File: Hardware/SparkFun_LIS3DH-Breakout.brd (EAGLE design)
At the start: 15.2 x 15.2 mm, 15 parts, among them U2 LIS3DH

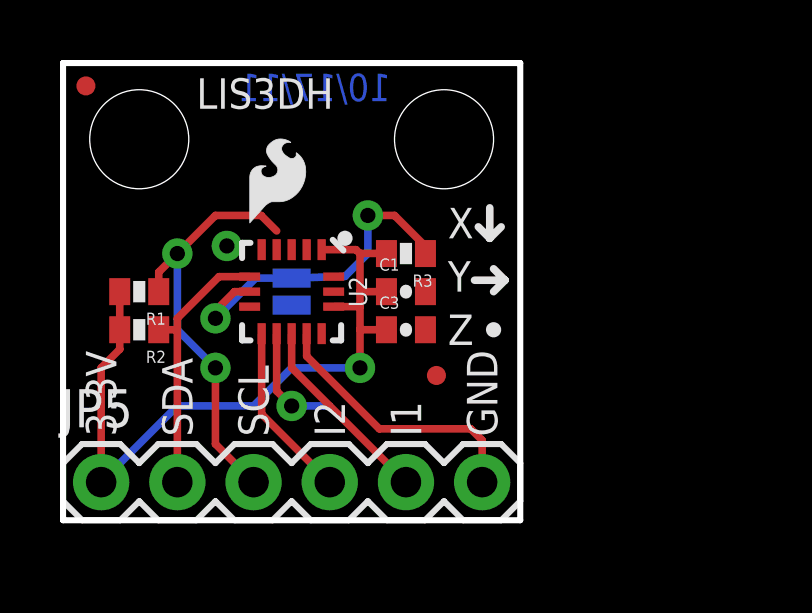
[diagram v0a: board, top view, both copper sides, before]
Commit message: Finished design for proto 1
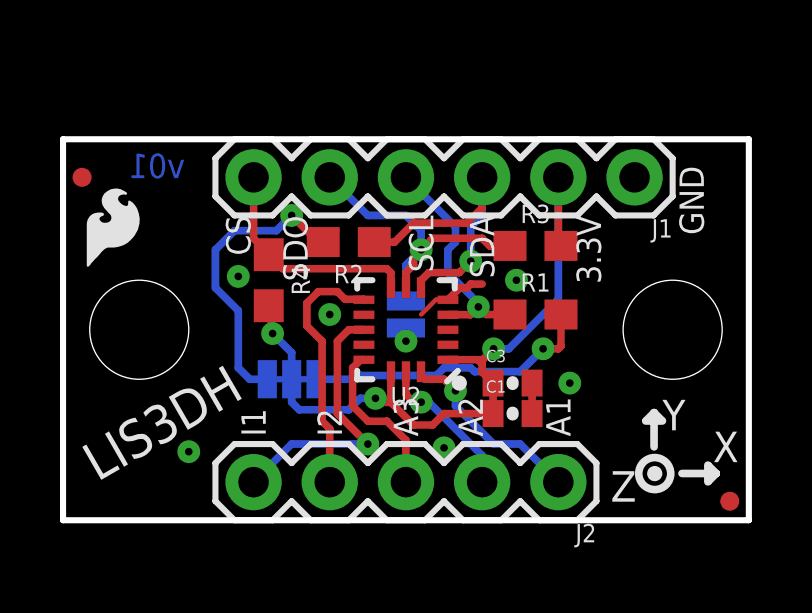
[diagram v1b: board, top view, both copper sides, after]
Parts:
- removed JP1: LOGO-SFESK, SparkFun:SFE-LOGO-FLAME
- removed JP5: (no value), SparkFun:1X06
- removed U$2: CREATIVE_COMMONS, SparkFun:CREATIVE_COMMONS
- added FRAME2: FRAME-LETTER, SparkFun-Aesthetics:CREATIVE_COMMONS
- added J1: (no value), SparkFun-Connectors:1X06
- added J2: (no value), SparkFun-Connectors:1X05
- added LOGO1: SFE_LOGO_FLAME.1_INCH, SparkFun-Aesthetics:SFE_LOGO_FLAME_.1
- added R4: 10k, SparkFun-Resistors:0603
- added SJ2: (no value), TestAperatures:PAD-JUMPER-3-3OF3_NC_BY_TRACE_YES_SILK_FULL_BOX
- R1, R2: value 10k -> 4.7k; device SparkFun:0402-RES -> SparkFun-Resistors:0603
- R3: device SparkFun:0402-RES -> SparkFun-Resistors:0603
- moved U$1 16.7 mm to (20.8, 1.65)
- moved R1 13.2 mm to (15.7, 6.86), turned to 0 degrees
- moved JP2 10.6 mm to (22.2, 0.64)
- moved JP4 9.92 mm to (20.3, 6.35)
- moved R2 7.57 mm to (9.53, 9.27)
- moved JP3 6.35 mm to (2.54, 6.35)
- moved C1 5.40 mm to (15.0, 3.56)
- moved R3 4.33 mm to (15.7, 9.14), turned to 0 degrees
- moved U2 4.02 mm to (11.4, 6.35), turned to 180 degrees
- moved C3 3.98 mm to (15.0, 4.57)
- moved SJ1 3.89 mm to (11.4, 6.86)
- moved JP6 3.05 mm to (0.64, 11.4)
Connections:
- new net ADC1: J2.1, U2.16
- new net ADC2: J2.2, U2.15
- new net ADC3: J2.3, U2.13
- new net CS: J1.6, R4.1, U2.8
- new net N$1: R2.2, SJ2.1
- new net N$2: R1.2, SJ2.3
- net 3.3V: now also J1.2, R4.2, SJ2.2; no longer JP5.1, R1.2, R2.2
- net GND: now also J1.1; no longer JP5.6
- net INT1: now also J2.5; no longer JP5.5
- net INT2: now also J2.4; no longer JP5.4
- net SA0: now also J1.5
- net SCL: now also J1.4; no longer JP5.3
- net SDA: now also J1.3; no longer JP5.2
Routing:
- net N$1: track 0.00 -> 9.81 mm, vias 0 -> 1
- net N$2: track 0.00 -> 9.78 mm, vias 0 -> 1
- net GND: track 13.0 -> 4.03 mm, vias 2 -> 7
- net CS: track 0.00 -> 7.61 mm
- net ADC1: track 0.00 -> 6.47 mm, vias 0 -> 1
- net SCL: track 14.2 -> 7.81 mm, vias 2 -> 1
- net ADC3: track 0.00 -> 5.41 mm
- net ADC2: track 0.00 -> 5.03 mm, vias 0 -> 1
- net INT1: track 6.53 -> 9.23 mm, vias 0 -> 1
- net INT2: track 5.89 -> 8.46 mm
- net SDA: track 9.07 -> 10.2 mm, vias 0 -> 1
- net 3.3V: track 25.5 -> 24.8 mm, vias 1 -> 3
- net SA0: track 11.6 -> 11.0 mm, vias 2 -> 1
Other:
- board size 15.2 x 15.2 mm -> 22.9 x 12.7 mm
- board text added: "A1"
- board text added: "A2"
- board text added: "A3"
- board text added: "ADR"
- board text added: "CS"
- board text added: "Marshall Taylor"
- board text added: "PU EN"
- board text added: "SCL SCK"
- board text added: "SDA SDI"
- board text added: "SDO"
- board text added: "v01"
- board text removed: "10/17/11"
- board text removed: "SA0"
